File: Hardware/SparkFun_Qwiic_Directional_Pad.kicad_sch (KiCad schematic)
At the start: 36 parts, among them J1 Qwiic_RA, J2 Conn_01x04, J3 Qwiic_RA, J5 I2C, SW2 Nav Switch, U4 PCA9557PW

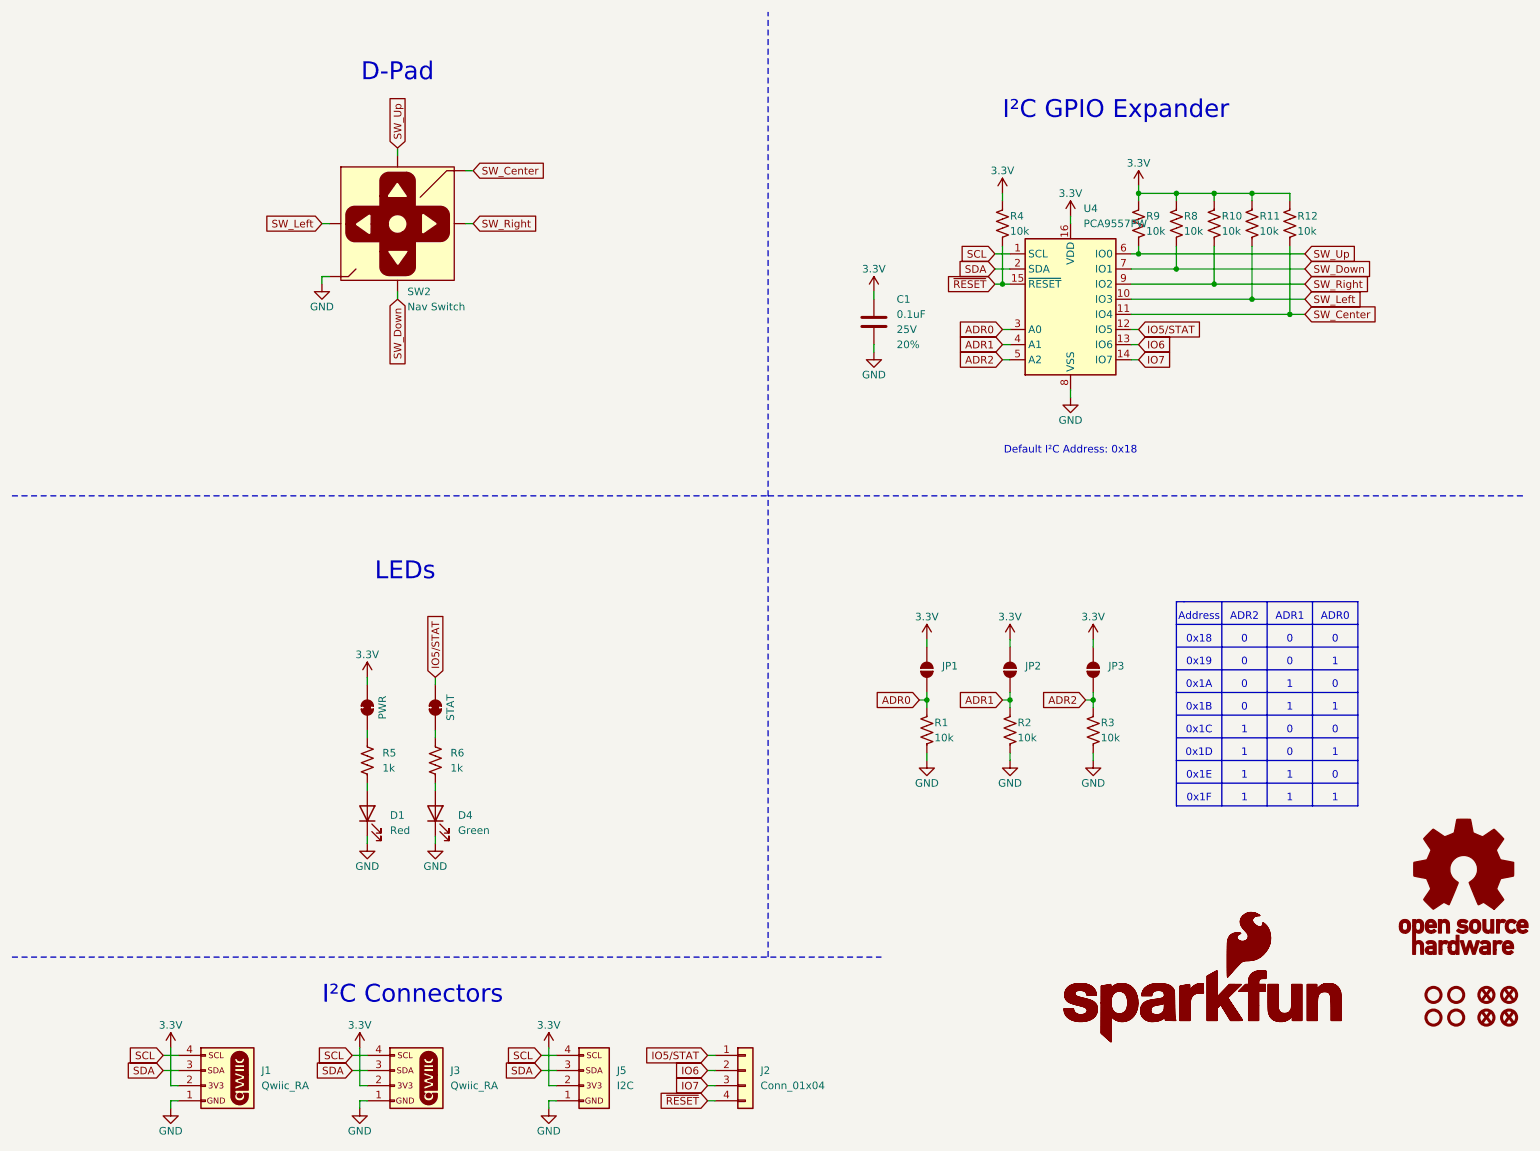
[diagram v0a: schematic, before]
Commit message: Fix page names.
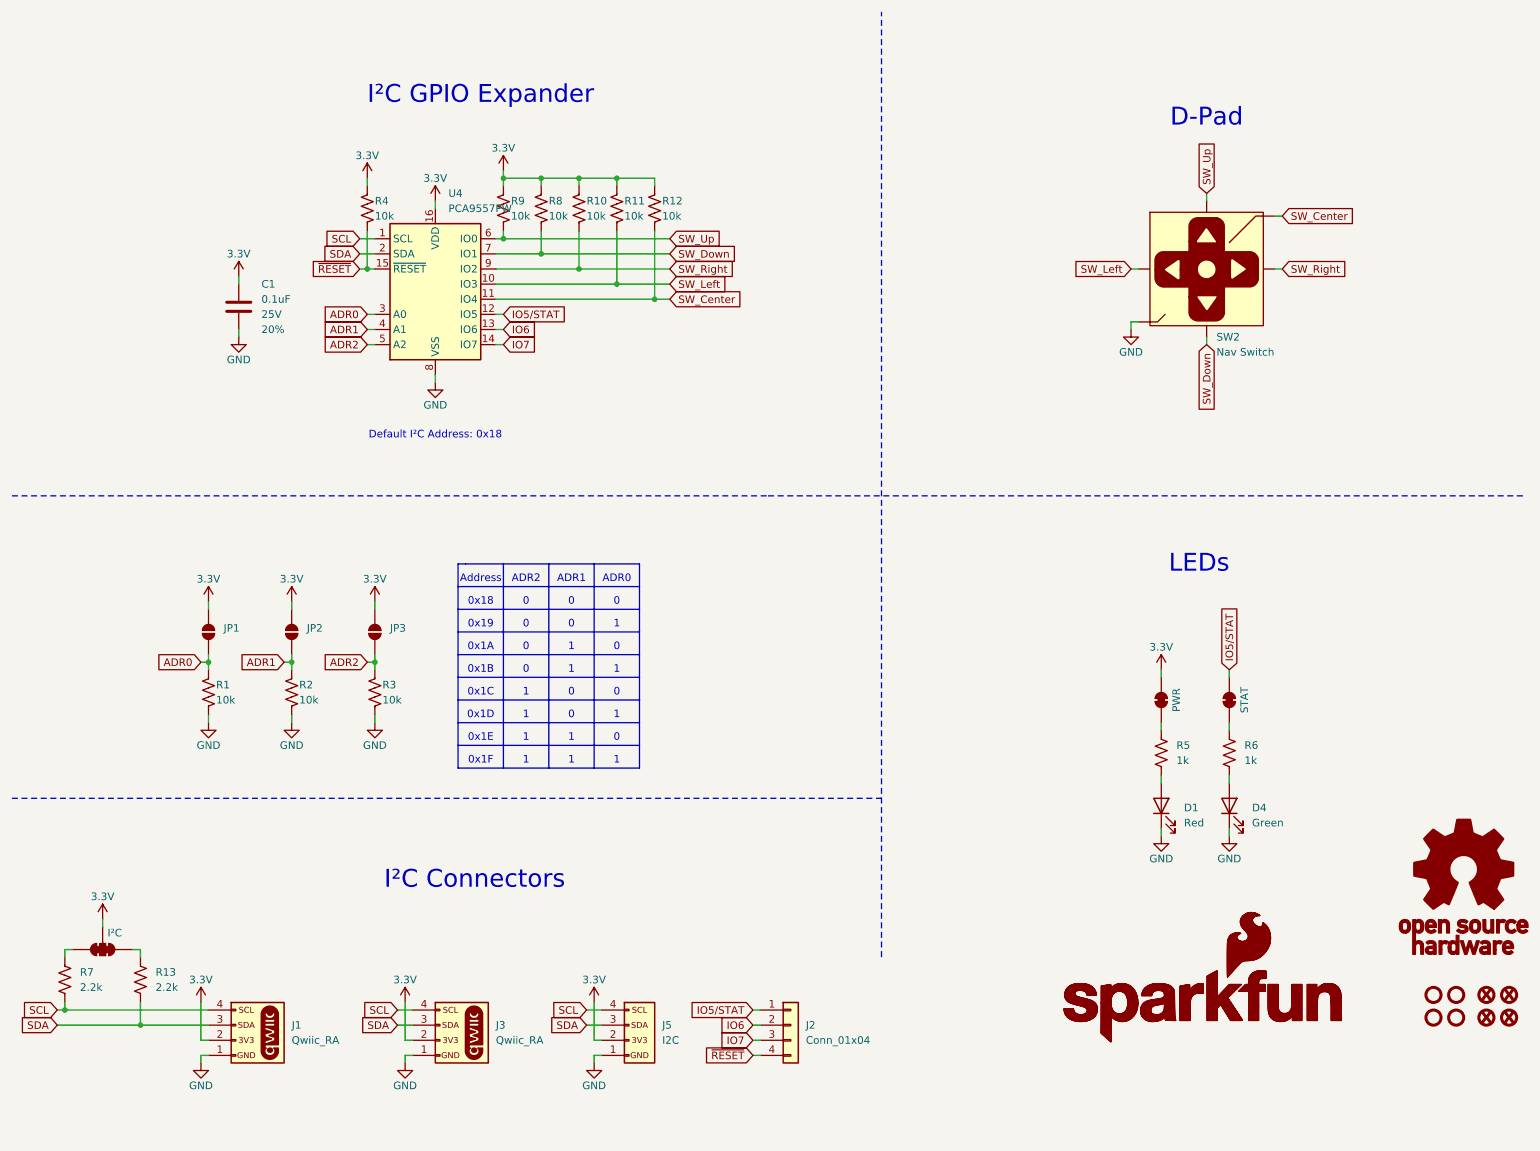
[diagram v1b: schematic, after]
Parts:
- added JP6: I²C, SparkFun-Jumper:Jumper_3_NC-2_Trace, symbol SparkFun-Jumper:SolderJumper_3_Bridged123
- added R13, R7: 2.2k, SparkFun-Resistor:R_0603_1608Metric, symbol SparkFun-Resistor:2.2k_0603
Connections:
- net 3.3V: now also JP6.2 (C)
- net SCL: now also R7.2
- net SDA: now also R13.2
- new net: JP6.1 (A), R13.1
- new net: JP6.3 (B), R7.1
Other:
- title: RTK Postcard Portable Shield -> SparkFun Qwiic Directional Pad
- moved on the sheet: C1, D1, D4, J1, J2, J3, J5, JP1, JP2, JP3, R1, R10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
